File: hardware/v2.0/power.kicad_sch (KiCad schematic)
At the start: 57 parts, among them U1 ECP5U-25F-CABGA256, U2 LTC3407AEDD-2_PBF, U3 TLV62569DBV

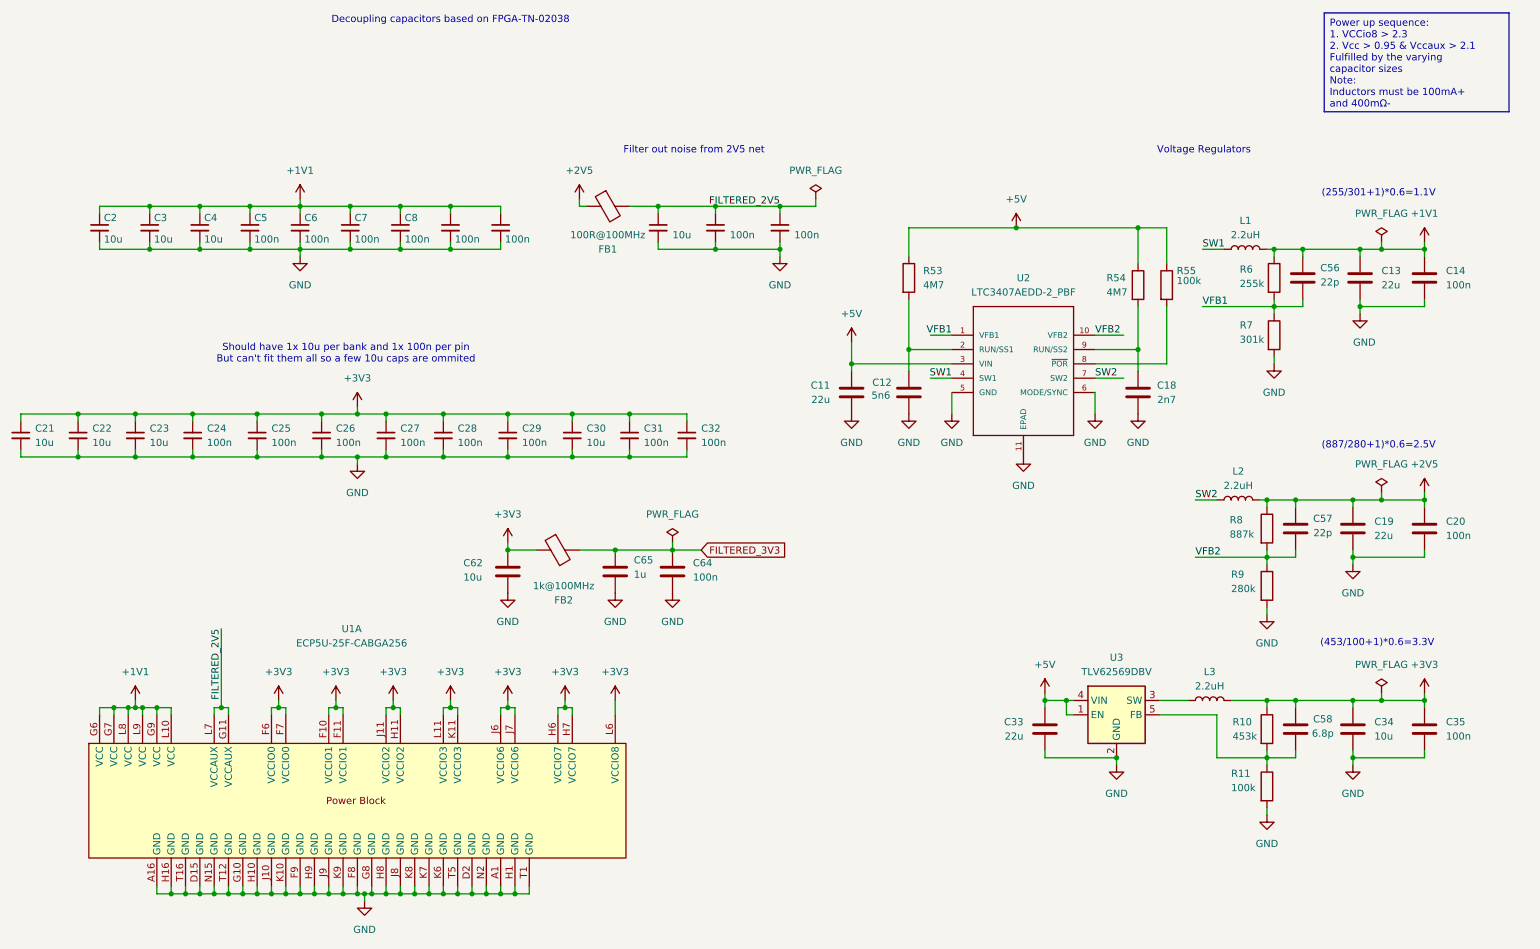
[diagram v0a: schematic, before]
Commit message: TLV62569DBVR Voltage Regulator
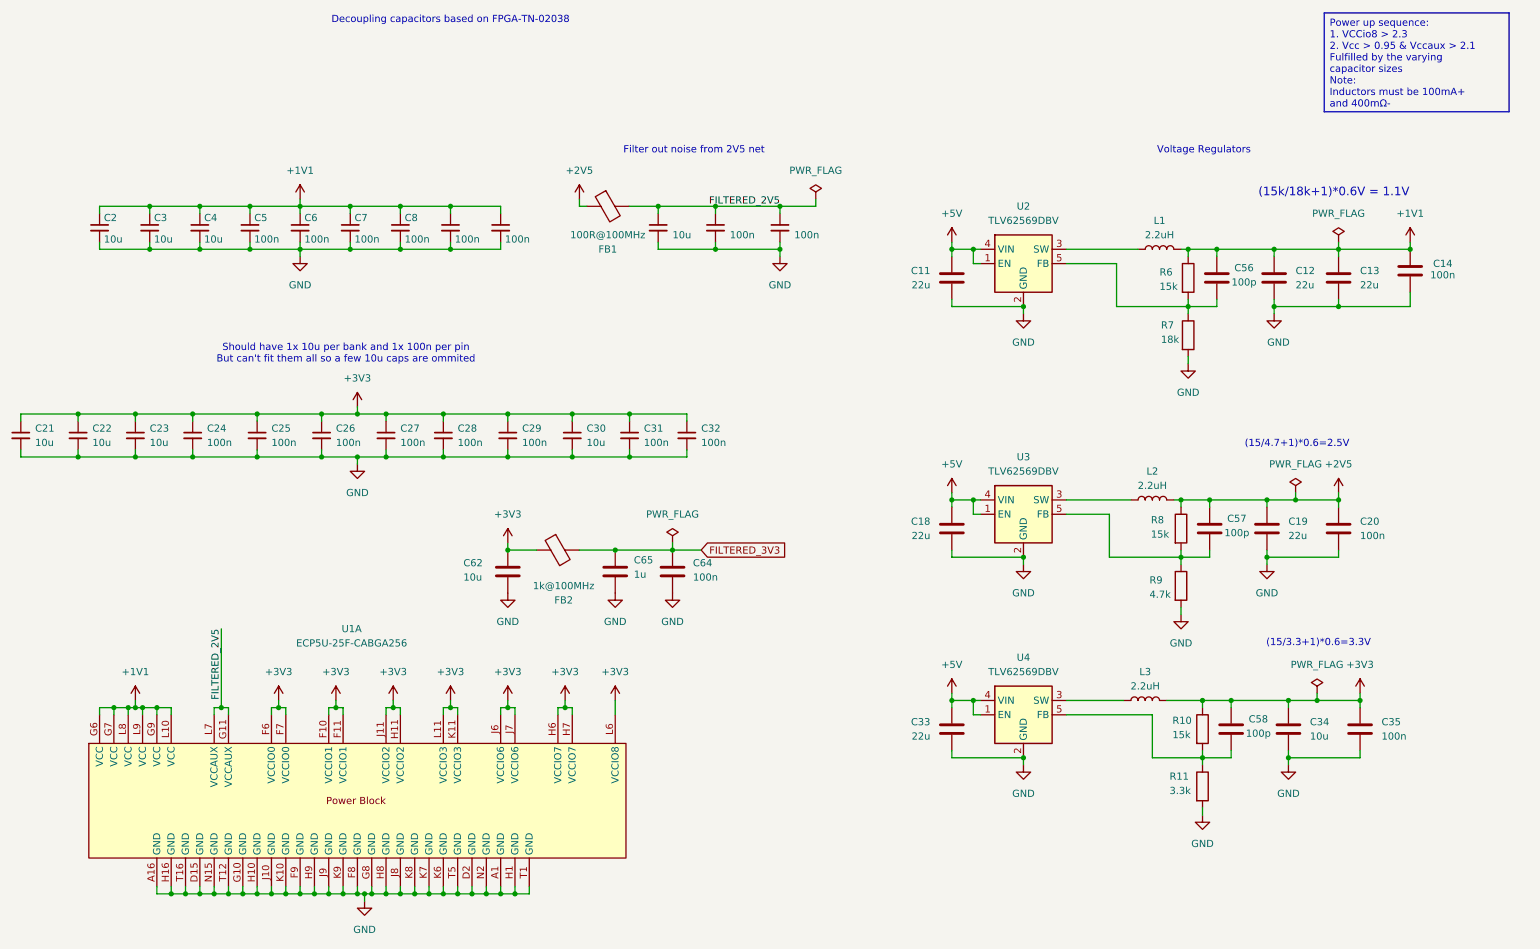
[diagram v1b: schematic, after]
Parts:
- removed R53, R54: 4M7, Resistor_SMD:R_0402_1005Metric, symbol Device:R
- removed R55: 100k, Resistor_SMD:R_0402_1005Metric, symbol Device:R
- removed U2: LTC3407AEDD-2_PBF, LTC3407AEDD-2_PBF:DFN-10_DD, symbol LTC3407AEDD-2_PBF:LTC3407AEDD-2_PBF
- added U2, U3: TLV62569DBV, Package_TO_SOT_SMD:SOT-23-5, symbol Regulator_Switching:TLV62569DBV
- C12: value 5n6 -> 22u; footprint Capacitor_SMD:C_0402_1005Metric -> Capacitor_SMD:C_0603_1608Metric; LCSC Link https://www.lcsc.com/product-detail/C307435.html -> https://lcsc.com/product-detail/Multilayer-Ceramic-Capacito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; LCSC Part # C3878619 -> C59461; MANUFACTURER muRata -> Samsung Electro-Mechanics; MANUFACTURER_PART_NUMBER GRM1555C1H562GE01D -> CL10A226MQ8NRNC; Manufactuer Part Number CL05B562KB5NNNC -> CL10A226MQ8NRNC
- C18: value 2n7 -> 22u; footprint Capacitor_SMD:C_0402_1005Metric -> Capacitor_SMD:C_0603_1608Metric; LCSC Link https://www.lcsc.com/product-detail/C84704.html -> https://lcsc.com/product-detail/Multilayer-Ceramic-Capacito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; LCSC Part # C84704 -> C59461; MANUFACTURER_PART_NUMBER CL05B272KB5NNNC -> CL10A226MQ8NRNC; Manufactuer Part Number CL05B272KB5NNNC -> CL10A226MQ8NRNC
- C56, C57: value 22p -> 100p; LCSC Link https://www.lcsc.com/product-detail/C70464.html -> https://www.lcsc.com/product-detail/C26409.html; LCSC Part # C70464 -> C26409; MANUFACTURER_PART_NUMBER CL05C220JB5NNNC -> CL05C101JB5NNNC; Manufactuer Part Number CL05C220JB5NNNC -> CL05C101JB5NNNC
- C58: value 6.8p -> 100p; LCSC Link https://www.lcsc.com/product-detail/C318598.html -> https://www.lcsc.com/product-detail/C26409.html; LCSC Part # C318598 -> C26409; MANUFACTURER_PART_NUMBER CL05C6R8CB5NNNC -> CL05C101JB5NNNC; Manufactuer Part Number CL05C6R8CB5NNNC -> CL05C101JB5NNNC
- R10: value 453k -> 15k; LCSC Link https://www.lcsc.com/product-detail/C27009.html -> https://lcsc.com/product-detail/Chip-Resistor-Surface-Mount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; LCSC Part # C27009 -> C25756; MANUFACTURER_PART_NUMBER 0402WGF4533TCE -> 0402WGF1502TCE; Manufactuer Part Number 0402WGF4533TCE -> 0402WGF1502TCE
- R11: value 100k -> 3.3k; LCSC Link https://www.lcsc.com/product-detail/C25741.html -> https://lcsc.com/product-detail/Chip-Resistor-Surface-Mount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; LCSC Part # C25741 -> C25890; MANUFACTURER_PART_NUMBER 0402WGF1003TCE -> 0402WGF3301TCE; Manufactuer Part Number 0402WGF1003TCE -> 0402WGF3301TCE
- R6: value 255k -> 15k; LCSC Link https://www.lcsc.com/product-detail/C270623.html -> https://lcsc.com/product-detail/Chip-Resistor-Surface-Mount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; LCSC Part # C270623 -> C25756; MANUFACTURER_PART_NUMBER 0402WGF2553TCE -> 0402WGF1502TCE; Manufactuer Part Number 0402WGF2553TCE -> 0402WGF1502TCE
- R7: value 301k -> 18k; LCSC Link https://www.lcsc.com/product-detail/C25775.html -> https://www.lcsc.com/product-detail/C25762.html; LCSC Part # C25775 -> C25762; MANUFACTURER_PART_NUMBER 0402WGF3013TCE -> 0402WGF1802TCE; Manufactuer Part Number 0402WGF3013TCE -> 0402WGF1802TCE
- R8: value 887k -> 15k; LCSC Link https://www.lcsc.com/product-detail/C423127.html -> https://lcsc.com/product-detail/Chip-Resistor-Surface-Mount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; LCSC Part # C423127 -> C25756; MANUFACTURER_PART_NUMBER 0402WGF8873TCE -> 0402WGF1502TCE; Manufactuer Part Number 0402WGF8873TCE -> 0402WGF1502TCE
- R9: value 280k -> 4.7k; LCSC Link https://www.lcsc.com/product-detail/C46006.html -> https://lcsc.com/product-detail/Chip-Resistor-Surface-Mount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; LCSC Part # C46006 -> C25900; MANUFACTURER_PART_NUMBER 0402WGF2803TCE -> 0402WGF4701TCE; Manufactuer Part Number 0402WGF2803TCE -> 0402WGF4701TCE
- renumbered U3 to U4
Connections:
- net +1V1: now also C12.1
- net +5V: now also C18.1, U2.1 (EN), U2.4 (VIN), U3.1 (EN), U3.4 (VIN)
- net GND: now also C12.2, U2.2 (GND), U3.2 (GND); no longer C12.1
- net SW1: no longer names the net of L1.1
- net SW1: now also U2.3 (SW)
- net SW2: no longer names the net of L2.1
- net SW2: now also U3.3 (SW)
- net VFB1: no longer names the net of C56.2, R6.2, R7.1
- net VFB1: now also U2.5 (FB)
- net VFB2: no longer names the net of C57.2, R8.2, R9.1
- net VFB2: now also U3.5 (FB)
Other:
- note added: "(15/3.3+1)*0.6=3.3V"
- note added: "(15/4.7+1)*0.6=2.5V"
- note added: "(15k/18k+1)*0.6V = 1.1V"
- note removed: "(255/301+1)*0.6=1.1V"
- note removed: "(453/100+1)*0.6=3.3V"
- note removed: "(887/280+1)*0.6=2.5V"
- moved on the sheet: C11, C13, C14, C19, C20, C33, C34, C35, C56, C57, C58, L1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
